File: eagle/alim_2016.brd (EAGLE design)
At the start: 90 x 50 mm, 57 parts, among them J1 AVR_SPI_PRG_6PTH, J2 AVR_SPI_PRG_6PTH, U1 3.3V, U2 LM2678S-5.0, U4 LM2596S-ADJ, U5 ATTINY85-20SU, U6 ATMEGA328P_TQFP

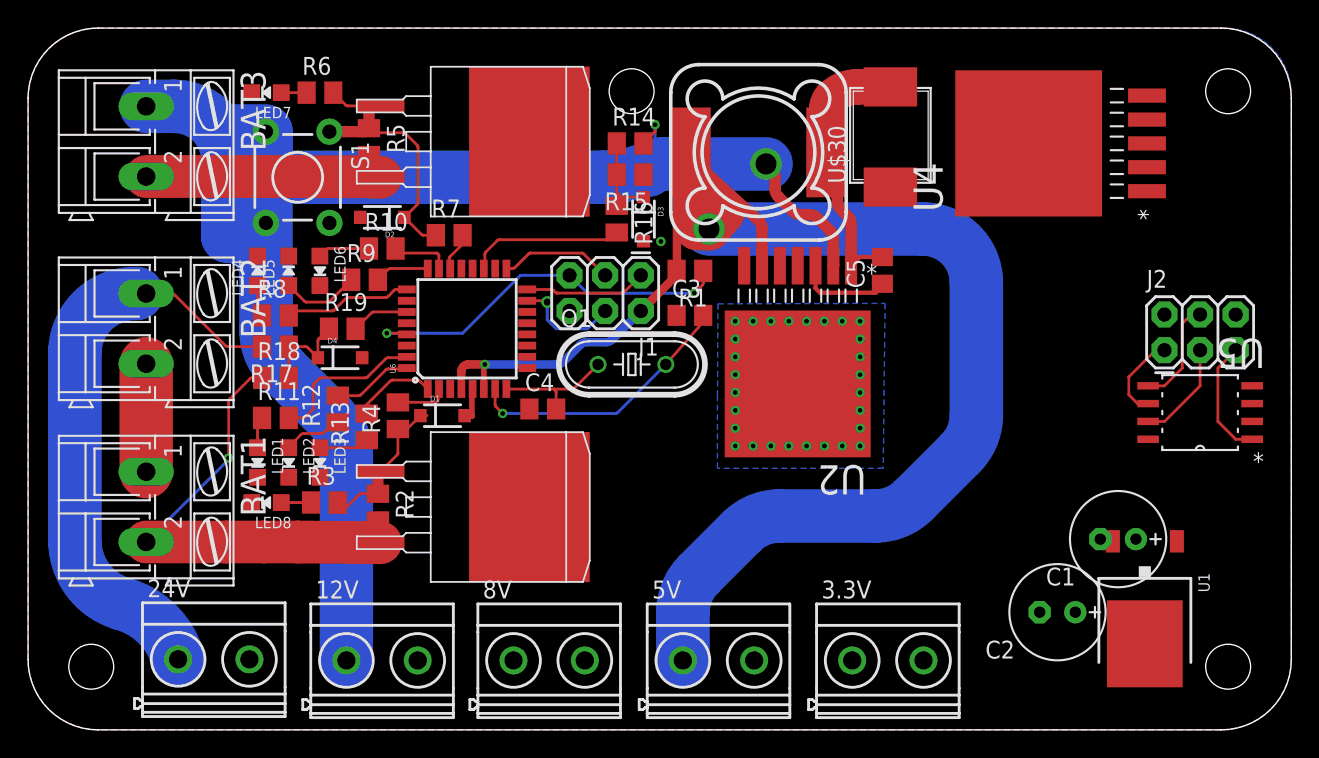
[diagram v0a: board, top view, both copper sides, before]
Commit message: rearrange stuff
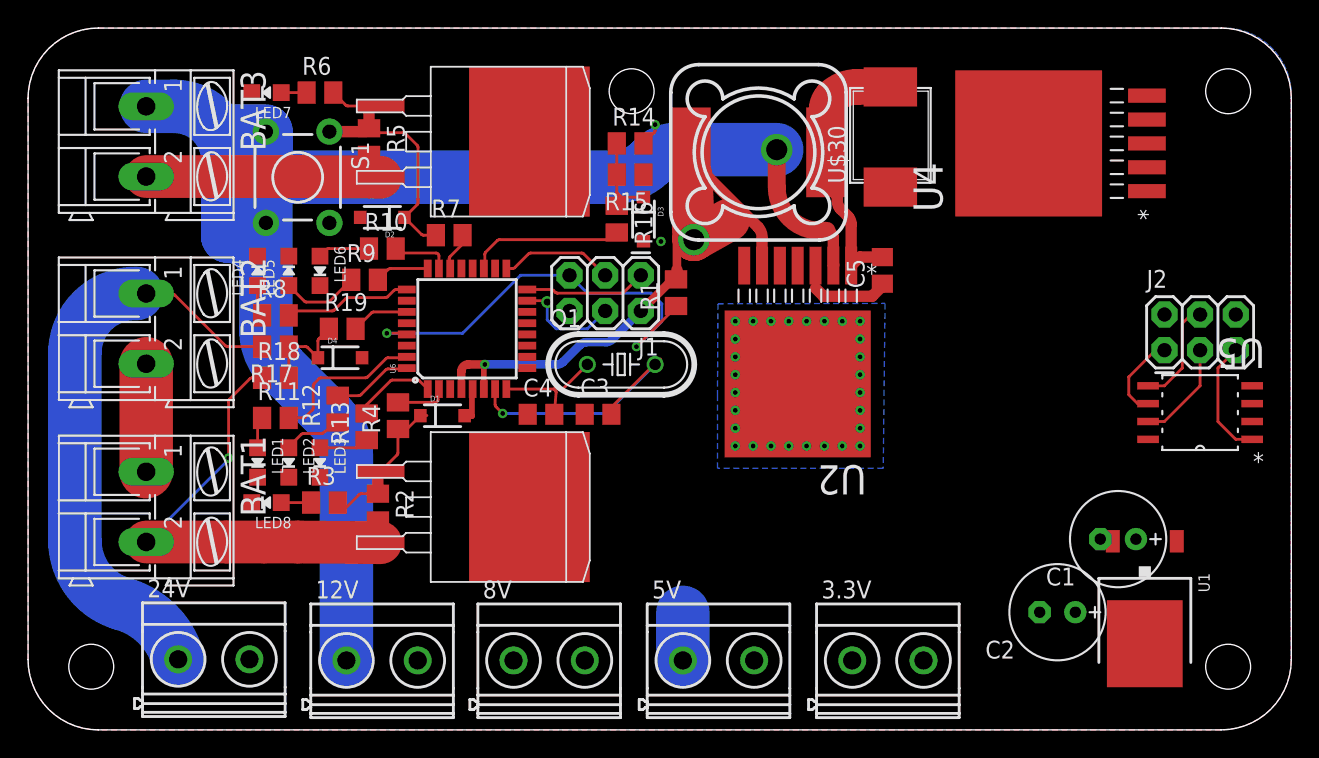
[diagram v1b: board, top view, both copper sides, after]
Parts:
- moved C3 9.62 mm to (40.6, 22.5)
- moved R1 1.84 mm to (46.2, 31.1), turned to 90 degrees
- moved Q1 0.76 mm to (42.3, 26.0)
- moved C4 0.40 mm to (36.5, 22.5)
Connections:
- net N$29 renamed SW
- net N$30 renamed BOOST
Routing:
- net 5.0V: track 107.3 -> 51.8 mm
- net RESET: track 27.4 -> 31.5 mm
